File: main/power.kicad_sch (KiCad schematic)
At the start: 8 parts, among them J3 USB_B_Micro, J4 external_power, U100 AP1117-33

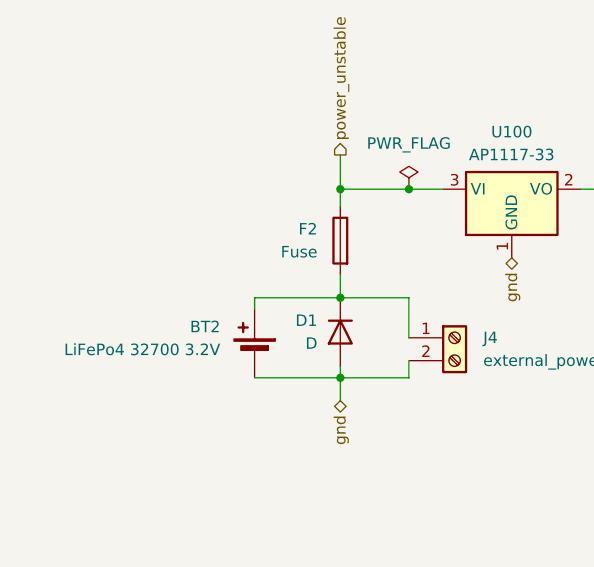
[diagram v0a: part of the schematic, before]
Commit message: Battery connection changed
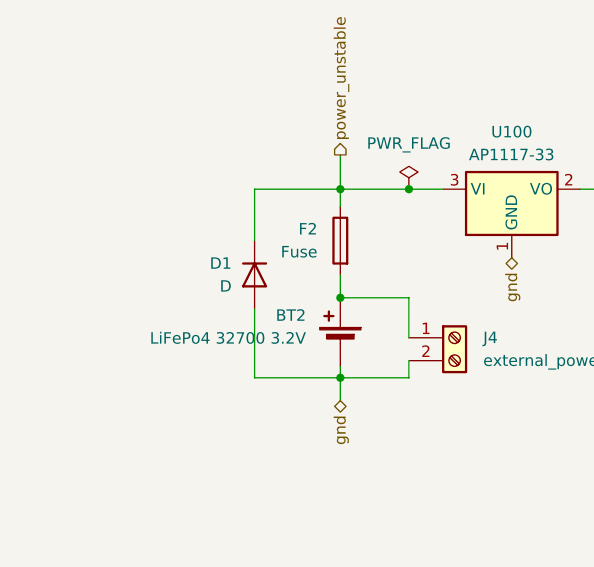
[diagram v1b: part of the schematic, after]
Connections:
- net power_unstable: now also D1.1 (K)
- net at BT2.1 (+), F2.2, J4.1 (Pin_1): no longer D1.1 (K)
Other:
- moved on the sheet: BT2, D1
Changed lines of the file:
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@@
+    (stroke (width 0) (type default))
+  )
+  (wire (pts (xy 47.625 41.91) (xy 47.625 47.625))
     (stroke (width 0) (type default))
   )
@@
     (stroke (width 0) (type default))
   )
-  (wire (pts (xy 57.15 43.815) (xy 57.15 41.91))
+  (wire (pts (xy 57.15 41.91) (xy 57.15 43.815))
     (stroke (width 0) (type default))
   )
@@
     (stroke (width 0) (type default))
   )
+  (wire (pts (xy 47.625 55.245) (xy 47.625 62.865))
+    (stroke (width 0) (type default))
+  )
   (wire (pts (xy 83.82 41.91) (xy 90.17 41.91))
     (stroke (width 0) (type default))
@@
     (stroke (width 0) (type default))
   )
-  (wire (pts (xy 47.625 53.975) (xy 57.15 53.975))
-    (stroke (width 0) (type default))
-  )
   (wire (pts (xy 138.43 87.63) (xy 128.27 87.63))
     (stroke (width 0) (type default))
@@
     (stroke (width 0) (type default))
   )
-  (wire (pts (xy 47.625 53.975) (xy 47.625 55.245))
-    (stroke (width 0) (type default))
-  )
   (wire (pts (xy 138.43 90.17) (xy 132.08 90.17))
     (stroke (width 0) (type default))
@@
     (stroke (width 0) (type default))
   )
+  (wire (pts (xy 47.625 41.91) (xy 57.15 41.91))
+    (stroke (width 0) (type default))
+  )
   (wire (pts (xy 177.8 43.18) (xy 180.975 43.18))
     (stroke (width 0) (type default))
@@
     (effects (font (size 1.27 1.27)) (justify right))
   )
-  (symbol (lib_id "Device:Battery_Cell") (at 47.625 60.325 0) (mirror y) (unit 1)
+  (symbol (lib_id "Device:Battery_Cell") (at 57.15 59.055 0) (mirror y) (unit 1)
     (in_bom yes) (on_board yes) (dnp no)
-    (property "Reference" "BT2" (at 43.815 57.2135 0)
-      (effects (font (size 1.27 1.27)) (justify left))
-    )
-    (property "Value" "LiFePo4 32700 3.2V" (at 43.815 59.7535 0)
-      (effects (font (size 1.27 1.27)) (justify left))
-    )
-    (property "Footprint" "" (at 47.625 58.801 90)
-      (effects (font (size 1.27 1.27)) hide)
-    )
-    (property "Datasheet" "~" (at 47.625 58.801 90)
+    (property "Reference" "BT2" (at 53.34 55.9435 0)
+      (effects (font (size 1.27 1.27)) (justify left))
+    )
+    (property "Value" "LiFePo4 32700 3.2V" (at 53.34 58.4835 0)
+      (effects (font (size 1.27 1.27)) (justify left))
+    )
+    (property "Footprint" "" (at 57.15 57.531 90)
+      (effects (font (size 1.27 1.27)) hide)
+    )
+    (property "Datasheet" "~" (at 57.15 57.531 90)
       (effects (font (size 1.27 1.27)) hide)
     )
@@
     )
   )
-  (symbol (lib_id "Device:D") (at 57.15 57.785 90) (mirror x) (unit 1)
+  (symbol (lib_id "Device:D") (at 47.625 51.435 90) (mirror x) (unit 1)
     (in_bom yes) (on_board yes) (dnp no)
-    (property "Reference" "D1" (at 54.61 56.515 90)
-      (effects (font (size 1.27 1.27)) (justify left))
-    )
-    (property "Value" "D" (at 54.61 59.055 90)
-      (effects (font (size 1.27 1.27)) (justify left))
-    )
-    (property "Footprint" "" (at 57.15 57.785 0)
-      (effects (font (size 1.27 1.27)) hide)
-    )
-    (property "Datasheet" "~" (at 57.15 57.785 0)
-      (effects (font (size 1.27 1.27)) hide)
-    )
-    (property "Sim.Device" "D" (at 57.15 57.785 0)
-      (effects (font (size 1.27 1.27)) hide)
-    )
-    (property "Sim.Pins" "1=K 2=A" (at 57.15 57.785 0)
-      (effects (font (size 1.27 1.27)) hide)
-    )
+    (property "Reference" "D1" (at 45.085 50.165 90)
+      (effects (font (size 1.27 1.27)) (justify left))
+    )
+    (property "Value" "D" (at 45.085 52.705 90)
+      (effects (font (size 1.27 1.27)) (justify left))
+    )
+    (property "Footprint" "" (at 47.625 51.435 0)
+      (effects (font (size 1.27 1.27)) hide)
+    )
+    (property "Datasheet" "~" (at 47.625 51.435 0)
+      (effects (font (size 1.27 1.27)) hide)
+    )
+    (property "Sim.Device" "D" (at 47.625 51.435 0)
+      (effects (font (size 1.27 1.27)) hide)
+    )
+    (property "Sim.Pins" "1=K 2=A" (at 47.625 51.435 0)
+      (effects (font (size 1.27 1.27)) hide)
+    )
